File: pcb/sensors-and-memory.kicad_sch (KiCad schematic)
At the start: 22 parts, among them J11 MSD-1-A, U3 BMP585, U4 W25Q128JVSIQ, U5 LSM6DSV320XTR

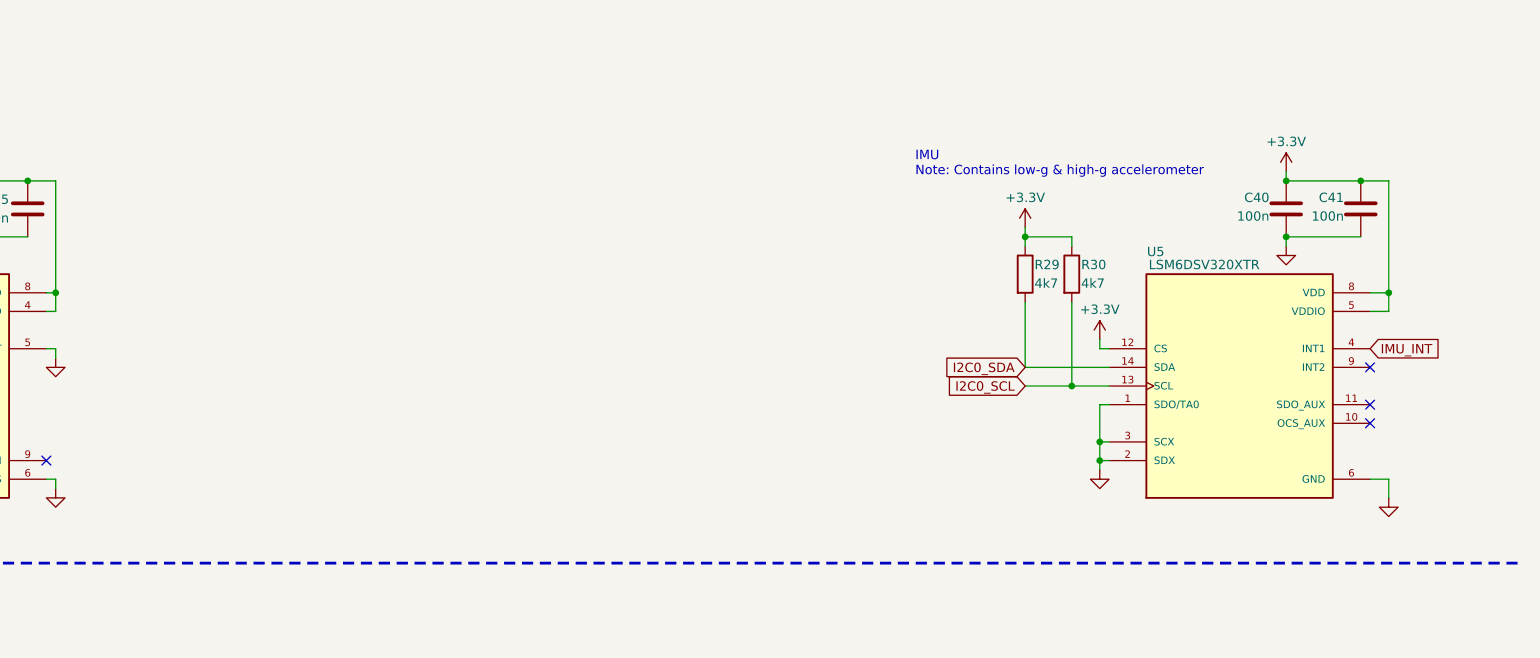
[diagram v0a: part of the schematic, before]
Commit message: PCB update
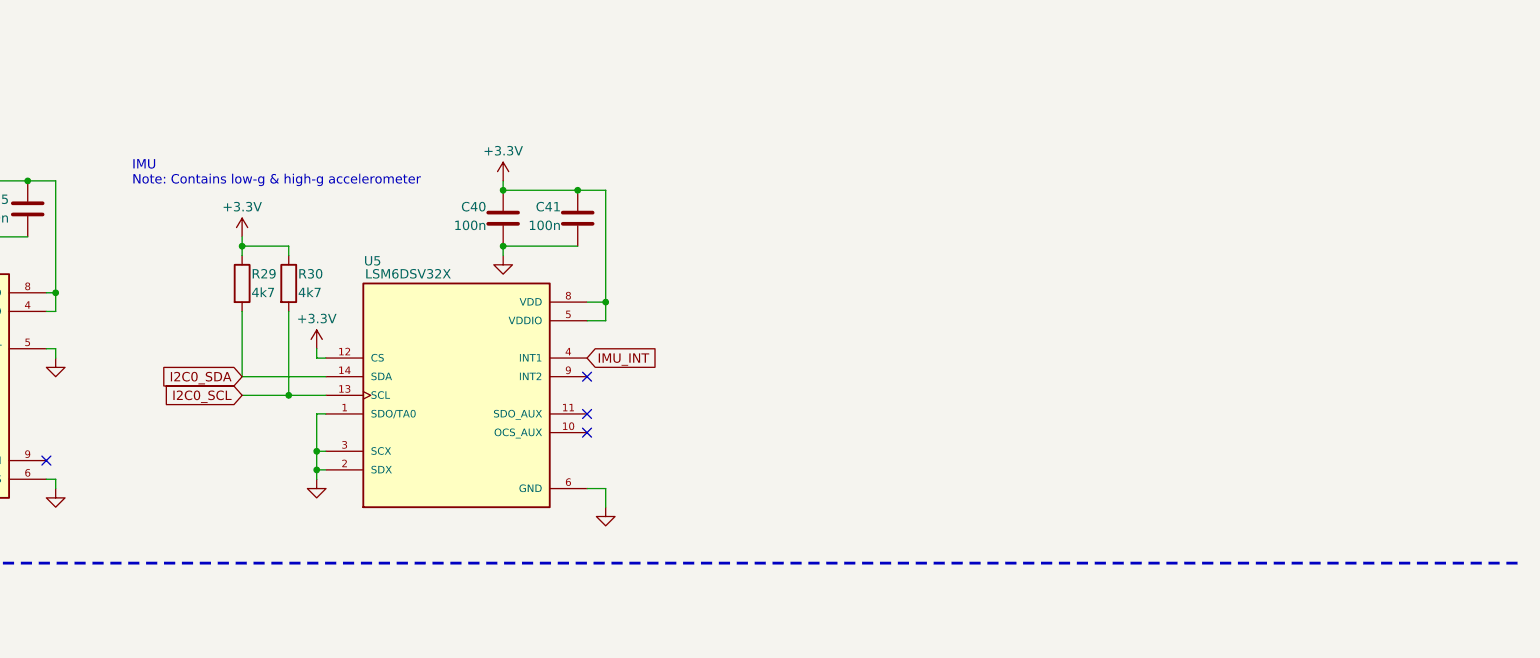
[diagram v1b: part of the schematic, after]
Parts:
- U5: value LSM6DSV320XTR -> LSM6DSV32X
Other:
- moved on the sheet: C40, C41, R29, R30, U5
